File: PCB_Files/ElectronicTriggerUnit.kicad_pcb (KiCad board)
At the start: 2 copper layers, 158.9 x 58.1 mm, 138 parts, among them IC1 ATTINY814-SSF, IC2 MCP1407-E_SN, IC3 MCP1407-E_SN, IC4 BU4S584G2-TR, IC5 ATTINY814-SSF, IC6 BU4S584G2-TR, IC7 ATTINY814-SSF, IC8 BU4S584G2-TR, IC9 MCP1407-E_SN, J1 Conn_01x04, J2 Conn_01x05, J3 Conn_01x04, J4 Conn_01x04, Q1 LC191PTDT, Q2 LKPT30102B-A01, Q3 SIR500DP-T1-RE3, Q4 SIR500DP-T1-RE3, Q5 LC191PTDT, Q6 LKPT30102B-A01, Q7 LC191PTDT, Q8 LKPT30102B-A01, Q9 SIR500DP-T1-RE3, U1 12v, U10 Gnd, U11 GndMotor, U13 12v, U14 GndMotor, U15 Gnd, U2 12v, U3 GndMotor, U4 Gnd, U5 Gnd, U6 12v, U7 SigIn, U8 Gnd, U9 12v

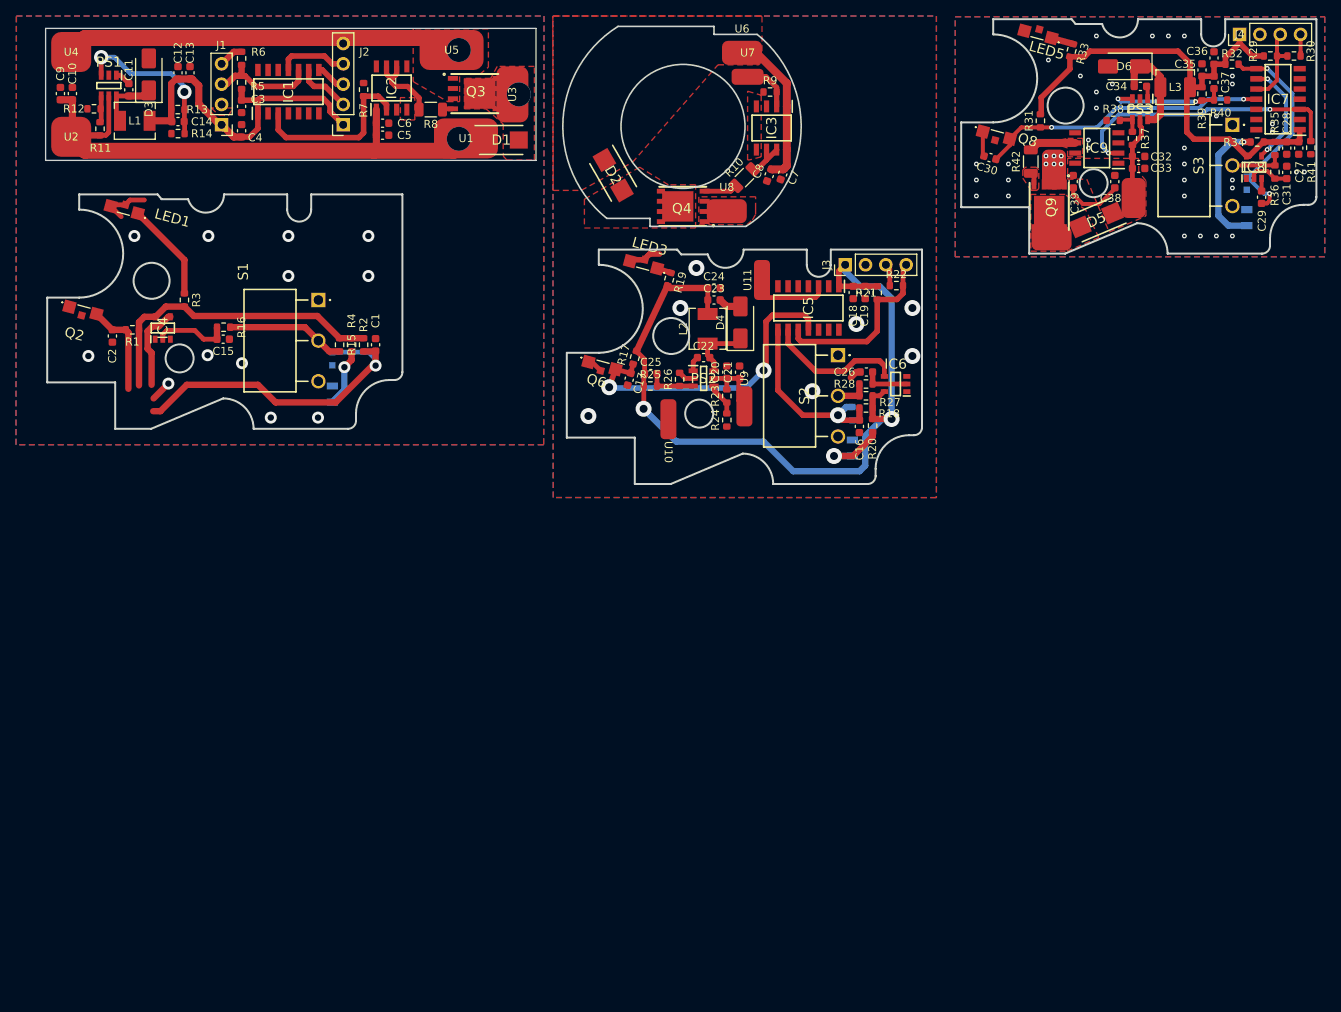
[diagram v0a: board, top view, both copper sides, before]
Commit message: stacked version
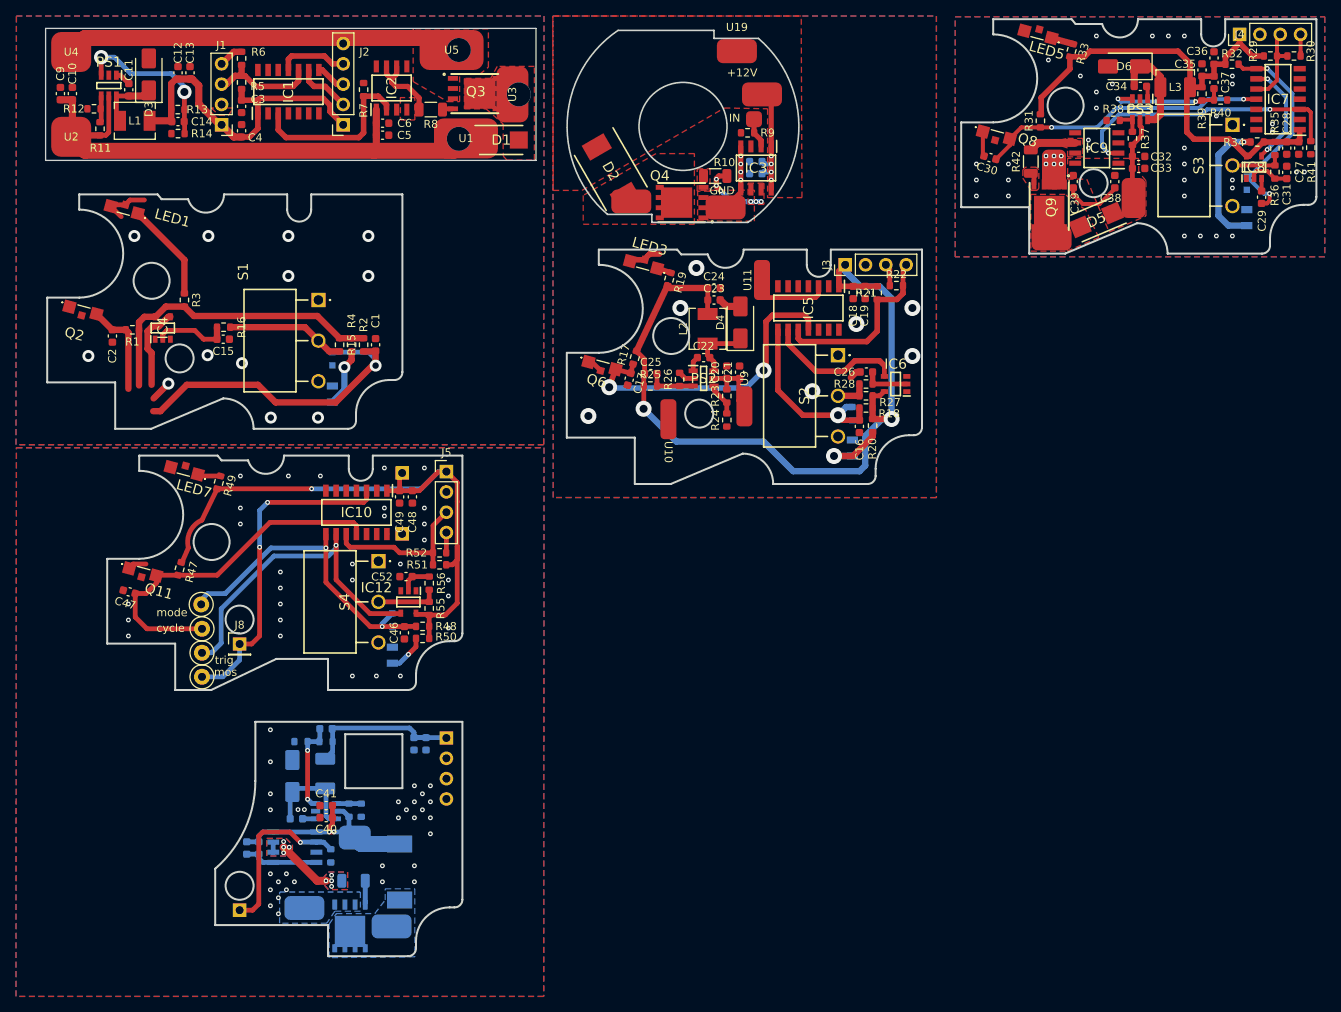
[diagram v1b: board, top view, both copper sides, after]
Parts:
- added C40: 10u/1206, Capacitor_SMD:C_0603_1608Metric, F.Cu at (99.7, 177.7)
- added C41: 10u/1206, Capacitor_SMD:C_0603_1608Metric, F.Cu at (99.7, 176.2)
- added C42: 22n, Capacitor_SMD:C_0603_1608Metric, B.Cu at (96.0, 177.8)
- added C43: 22u, Capacitor_SMD:C_0603_1608Metric, B.Cu at (112.2, 168.5)
- added C44: 22u, Capacitor_SMD:C_0603_1608Metric, B.Cu at (110.7, 168.5)
- added C45: 100p, Capacitor_SMD:C_0603_1608Metric, B.Cu at (99.7, 166.6)
- added C46: 10n, Capacitor_SMD:C_0603_1608Metric, F.Cu at (109.5, 154.6)
- added C47: 10n, Capacitor_SMD:C_0603_1608Metric, F.Cu at (75.1, 149.5)
- added C48: 1u, Capacitor_SMD:C_0603_1608Metric, F.Cu at (110.5, 137.6)
- added C49: 100n, Capacitor_SMD:C_0603_1608Metric, F.Cu at (108.9, 137.6)
- added C50: 1u, Capacitor_SMD:C_0603_1608Metric, B.Cu at (89.8, 181.5)
- added C51: 10u, Capacitor_SMD:C_0603_1608Metric, B.Cu at (91.3, 181.5)
- added C52: 100nf, Capacitor_SMD:C_0603_1608Metric, F.Cu at (109.7, 147.6)
- added D7: B340A, Diode_SMD:D_SMA, B.Cu at (95.5, 172.5)
- added D9: STPS5L60S, SamacSys:DIOM8059X265N, B.Cu at (108.9, 184.5)
- added IC10: ATTINY814-SSF, SamacSys:SOIC127P600X175-14N, F.Cu at (103.5, 139.6)
- added IC11: MCP1407-E_SN, SamacSys:SOIC127P600X175-8N, B.Cu at (95.8, 181.4)
- added IC12: BU4S584G2-TR, SamacSys:SOT95P280X125-5N, F.Cu at (110.0, 150.8)
- added J10: Conn_01x01, Connector_PinHeader_2.54mm:PinHeader_1x01_P2.54mm_Vertical, B.Cu at (109.2, 142.2)
- added J5: Conn_01x04, Connector_PinHeader_2.54mm:PinHeader_1x04_P2.54mm_Vertical, F.Cu at (114.8, 134.4)
- added J6: Conn_01x04, Connector_PinHeader_2.54mm:PinHeader_1x04_P2.54mm_Vertical, B.Cu at (114.8, 167.8)
- added J7: Conn_01x01, Connector_PinHeader_2.54mm:PinHeader_1x01_P2.54mm_Vertical, B.Cu at (88.9, 189.3)
- added J8: Conn_01x01, Connector_PinHeader_2.54mm:PinHeader_1x01_P2.54mm_Vertical, F.Cu at (88.9, 156.0)
- added J9: Conn_01x01, Connector_PinHeader_2.54mm:PinHeader_1x01_P2.54mm_Vertical, B.Cu at (109.2, 134.6)
- added L4: 10u/C2921170, Inductor_SMD:L_Chilisin_BMRA00040420, B.Cu at (99.6, 172.2)
- added LED7: LKIR30102C-A01, SamacSys:APA3010P3C, F.Cu at (82.0, 134.3)
- added LED8: XL-2012IRC-940, SamacSys:LEDC2012X105N, B.Cu at (108.0, 157.4)
- added PS4: AP5100WG-7, SamacSys:SOT95P285X140-6N, B.Cu at (99.7, 176.9)
- added Q10: LC191PTDT, SamacSys:AP1608P1CP22, B.Cu at (108.0, 153.0)
- added Q11: LKPT30102B-A01, SamacSys:APA3010P3C, F.Cu at (76.8, 147.0)
- added Q12: SIR500DP-T1-RE3, SamacSys:POWERPAKSO-8, B.Cu at (102.7, 191.3)
- added R43: 10k, Resistor_SMD:R_0603_1608Metric, B.Cu at (102.6, 176.8)
- added R44: 2k, Resistor_SMD:R_0603_1608Metric, B.Cu at (104.1, 176.8)
- added R45: 10k, Resistor_SMD:R_0603_1608Metric, B.Cu at (99.7, 168.2)
- added R46: 3.3k, Resistor_SMD:R_0603_1608Metric, B.Cu at (96.6, 168.2)
- added R47: 5K, Resistor_SMD:R_0603_1608Metric, F.Cu at (81.4, 146.6)
- added R48: 5K, Resistor_SMD:R_0603_1608Metric, F.Cu at (111.8, 153.8)
- added R49: 100R, Resistor_SMD:R_0603_1608Metric, F.Cu at (86.3, 135.8)
- added R50: 100R, Resistor_SMD:R_0603_1608Metric, F.Cu at (111.8, 155.3)
- added R51: 10k, Resistor_SMD:R_0603_1608Metric, F.Cu at (113.9, 146.1)
- added R52: 1k, Resistor_SMD:R_0603_1608Metric, F.Cu at (113.9, 144.6)
- added R53: 10k, Resistor_SMD:R_0603_1608Metric, B.Cu at (100.3, 182.5)
- added R54: 10R, Resistor_SMD:R_1206_3216Metric, B.Cu at (103.1, 185.6)
- added R55: 10K, Resistor_SMD:R_0603_1608Metric, F.Cu at (112.6, 151.6)
- added R56: 1K, Resistor_SMD:R_0603_1608Metric, F.Cu at (112.6, 148.4)
- added S4: Trigger, SamacSys:463092691402, F.Cu at (106.2, 145.7)
- added TP1: TestPoint, TestPoint:TestPoint_Loop_D1.80mm_Drill1.0mm_Beaded, F.Cu at (84.1, 151.1)
- added TP2: TestPoint, TestPoint:TestPoint_Loop_D1.80mm_Drill1.0mm_Beaded, F.Cu at (84.2, 160.1)
- added TP3: TestPoint, TestPoint:TestPoint_Loop_D1.80mm_Drill1.0mm_Beaded, F.Cu at (84.2, 157.1)
- added TP4: TestPoint, TestPoint:TestPoint_Loop_D1.80mm_Drill1.0mm_Beaded, F.Cu at (84.2, 154.1)
- added U12: 12v, SamacSys:Copper_Pad, B.Cu at (103.3, 180.2)
- added U16: GndMotor, SamacSys:Copper_Pad, B.Cu at (107.9, 191.3)
- added U17: Gnd, SamacSys:Copper_Pad, B.Cu at (97.0, 189.0)
- added U18: Gnd, SamacSys:Copper_Pad, F.Cu at (137.9, 100.7)
- added U19: 12v, SamacSys:Copper_Pad, F.Cu at (151.1, 81.9)
- C19: value 10n -> 100n
- C38, C5: value 0.1u -> 1u
- C39, C6: value 1u -> 10u
- C7: value 0.1u -> 1u; moved to B.Cu
- C8: value 1u -> 10u; moved to B.Cu
- D2: value SS24 -> STPS5L60S; footprint SamacSys:DIOM5436X247N -> SamacSys:DIOM8059X265N
- moved R9 5.82 mm to (152.4, 92.1)
- moved U6 5.77 mm to (154.2, 87.3)
- moved IC3 5.37 mm to (153.4, 96.5)
- moved U7 5.36 mm to (153.2, 90.4), turned to -90 degrees
- moved C7 3.69 mm to (153.4, 95.7), turned to 180 degrees
- moved R10 3.66 mm to (148.3, 97.5), turned to 0 degrees
- moved C8 1.69 mm to (153.4, 97.2), turned to 0 degrees
- moved D2 0.58 mm to (135.3, 96.9)
- moved Q4 0.49 mm to (144.2, 100.8)
- moved U8 0.49 mm to (149.7, 101.4)
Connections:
- LED5 pad 3: GND -> (no net)
- Q8 pad 3: GND -> (no net)
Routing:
- net +3.3V: track 250.0 -> 340.4 mm, vias 2 -> 3
- net /LayeredEtu/NMOS: track 0.00 -> 62.6 mm, vias 0 -> 3
- net /LayeredEtu/V_Cycle_In: track 0.00 -> 45.0 mm
- net /LayeredEtu/trigger_In: track 0.00 -> 40.6 mm, vias 0 -> 1
- net /LayeredEtu/Semi_Auto_In: track 0.00 -> 40.6 mm, vias 0 -> 2
- net +12V: track 110.1 -> 134.6 mm, vias 1 -> 7
- net GND: track 83.1 -> 103.3 mm, vias 60 -> 124
- net /LayeredEtu/updiRx: track 0.00 -> 19.8 mm
- net Net-(D7-K): track 0.00 -> 12.7 mm
- net /LayeredEtu/BuckStepDown/V_FB: track 0.00 -> 11.5 mm, vias 0 -> 2
- net Net-(IC11-OUT_1): track 0.00 -> 9.01 mm, vias 0 -> 8
- net Net-(S4-NO): track 0.00 -> 7.85 mm
- net Net-(IC3-OUT_1): track 5.34 -> 10.5 mm, vias 0 -> 6
- net Net-(LED8-Pad2): track 0.00 -> 4.85 mm, vias 0 -> 1
- net Net-(Q4-Pad4): track 4.21 -> 0.00 mm
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- added copper zone on B.Cu, net /LayeredEtu/pwr_motor
- added copper zone on B.Cu, net Net-(IC11-OUT_1)
- added copper zone on F.Cu, net Net-(IC11-OUT_1)
- added copper zone on F.Cu, net Net-(IC3-OUT_1)
- added copper zone on F.Cu, net Net-(Q4-Pad4)
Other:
- board size 158.9 x 58.1 mm -> 158.9 x 117.1 mm
- board text added: "+12V"
- board text added: "+BAT"
- board text added: "GND"
- board text added: "IN"
- board text added: "OUT"
- board text added: "cycle"
- board text added: "mode"
- board text added: "mos"
- board text added: "trig"
